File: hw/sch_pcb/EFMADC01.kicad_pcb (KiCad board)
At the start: 4 copper layers, 80 x 80 mm, 89 parts, among them J1 SM06B-GHS-TB, J2 SM03B-GHS-TB, J3 HEADER_1x01, J4 HEADER_2x03, J5 SM08B-GHS-TB, J6 SM06B-GHS-TB, SW1 KMT031 NGJ LHS C&K, U1 ISL21080DIH312Z-TK 1V25, U10 SN74LVC1G14QDCKRQ1, U11 SN74LVC1G14QDCKRQ1, U12 SN74LVC1G14QDCKRQ1, U13 VCNT2020, U2 OPA314, U3 MIC5504-3.3YM5, U4 PCF8583, U5 VCNT2020, U6 VCNT2020, U7 SHT31, U8 ATMEGA1284P-AU, U9 AT24CS64-SSHM, Y1 16MHz

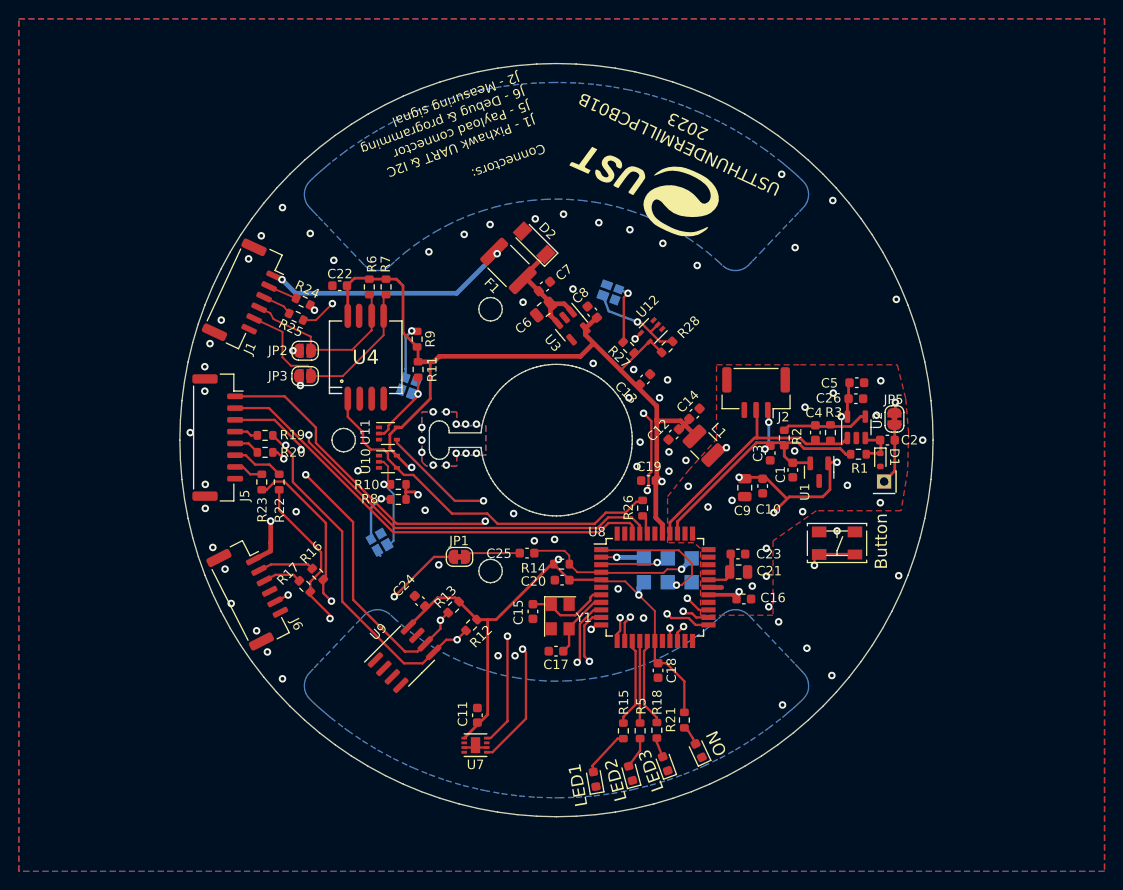
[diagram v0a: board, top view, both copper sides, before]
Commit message: Starting layout work.
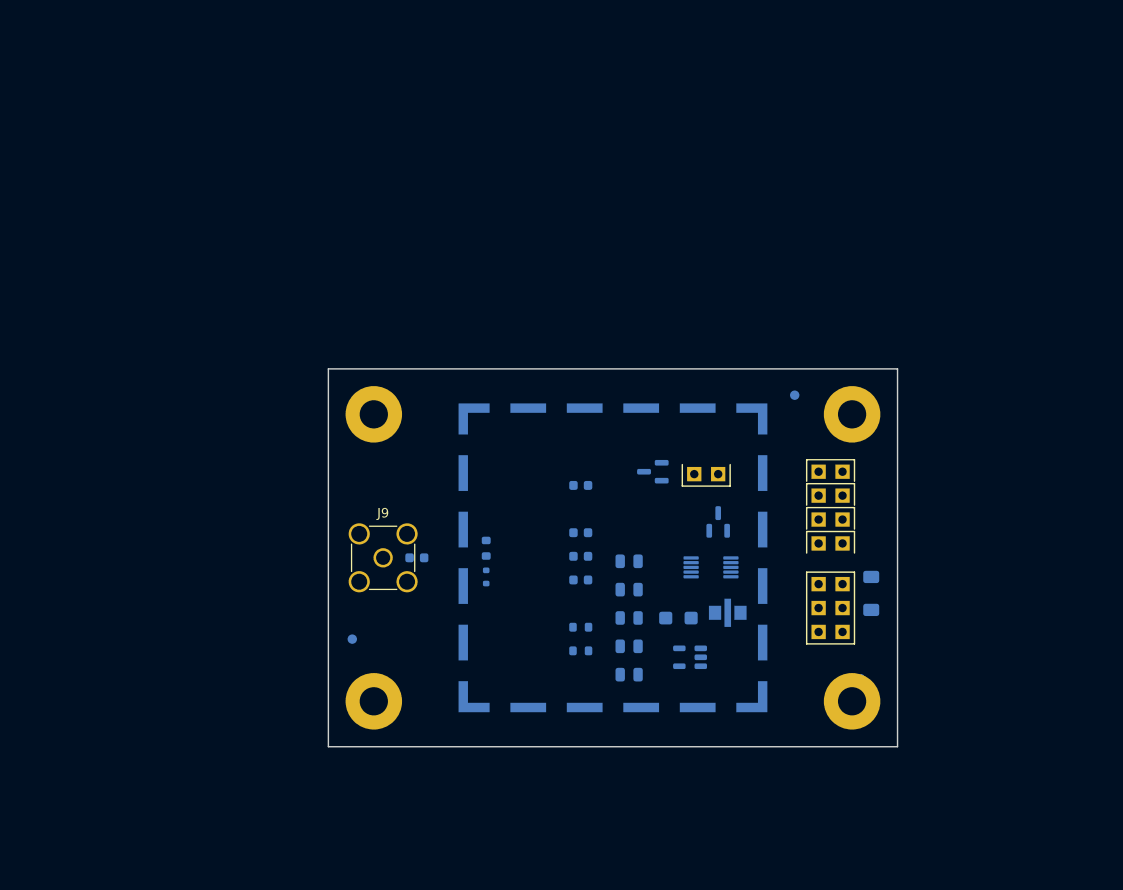
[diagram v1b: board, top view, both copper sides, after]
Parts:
- removed C13, C14, C16, C18, C19, C20, C22, C23, C24, C26: 100nF, Capacitor_SMD:C_0603_1608Metric
- removed C15, C17: 15 pF, Capacitor_SMD:C_0603_1608Metric
- removed C21: 10uF, Capacitor_SMD:C_0805_2012Metric
- removed C25: 4u7, Capacitor_SMD:C_0603_1608Metric
- removed D3: YELLOW, LED_SMD:LED_0603_1608Metric
- removed D4: BLUE, LED_SMD:LED_0603_1608Metric
- removed D5: GREEN, LED_SMD:LED_0603_1608Metric
- removed D6: RED, LED_SMD:LED_0603_1608Metric
- removed F1: 350mA, Fuse:Fuse_1812_4532Metric
- removed G1, G2: , MLAB_LOGA:UST
- removed J3: HEADER_1x01, Mlab_Pin_Headers:Straight_1x01
- removed JP2, JP3: SolderJumper_2_Open, Jumper:SolderJumper-2_P1.3mm_Open_RoundedPad1.0x1.5mm
- removed JP4: Jumper_2_Bridged, NetTie:NetTie-2_SMD_Pad0.5mm
- removed JP5: SolderJumper_2_Bridged, Jumper:SolderJumper-2_P1.3mm_Bridged_RoundedPad1.0x1.5mm
- removed L1: 10uH - LQH32CN100K23L, Inductor_SMD:L_1210_3225Metric
- removed R10, R11, R28: 4k7, Resistor_SMD:R_0603_1608Metric
- removed R12, R13, R14, R6, R7: 10k, Resistor_SMD:R_0603_1608Metric
- removed R15, R18, R21, R5: 2k2, Resistor_SMD:R_0603_1608Metric
- removed R16, R17, R22, R23, R24, R25, R26: 33R, Resistor_SMD:R_0603_1608Metric
- removed R19, R20, R27, R8, R9: 100R, Resistor_SMD:R_0603_1608Metric
- removed SW1: KMT031 NGJ LHS C&K, Mlab_SW:KMT031 NGJ LHS C&K
- removed U10, U11, U12: SN74LVC1G14QDCKRQ1, Package_TO_SOT_SMD:SOT-353_SC-70-5
- removed U13, U5, U6: VCNT2020, Mlab_IO:XDCR_VCNT2020
- removed U7: SHT31, Mlab_IO:DFN-8-1EP_2.4x2.4mm_Pitch0.5mm
- removed U8: ATMEGA1284P-AU, Package_QFP:TQFP-44_10x10mm_P0.8mm
- removed U9: AT24CS64-SSHM, Package_SO:SOIC-8_3.9x4.9mm_P1.27mm
- removed Y1: 16MHz, Mlab_XTAL:Crystal SMD CFPX-180
- added FID1: Fiducial, Fiducial:Fiducial_1mm_Mask2mm, B.Cu at (167.8, 87.7)
- added FID2: Fiducial, Fiducial:Fiducial_1mm_Mask2mm, B.Cu at (120.8, 113.6)
- added J7: HEADER_2x01_PARALLEL, Mlab_Pin_Headers:Straight_2x01, F.Cu at (171.6, 103.5)
- added J9: MCX, Connector_Coaxial:SMA_Amphenol_901-144_Vertical, F.Cu at (124.1, 105.0)
- added M1: RFShield_TwoPieces, RF_Shielding:Laird_Technologies_BMI-S-204-F_32.00x32.00mm, B.Cu at (148.5, 105.0)
- added M2: HOLE, Mlab_Mechanical:MountingHole_3mm, F.Cu at (123.1, 89.8)
- added M3: HOLE, Mlab_Mechanical:MountingHole_3mm, F.Cu at (173.9, 89.8)
- added M4: HOLE, Mlab_Mechanical:MountingHole_3mm, F.Cu at (123.1, 120.2)
- added M5: HOLE, Mlab_Mechanical:MountingHole_3mm, F.Cu at (173.9, 120.2)
- C1, C2, C3, C4, C5, D1, R1, R2, R3, U1, U2: moved to B.Cu
- C10, C11, C12: footprint Capacitor_SMD:C_0603_1608Metric -> Capacitor_SMD:C_0805_2012Metric; moved to B.Cu
- C6: value 10uF -> 1uF; footprint Capacitor_SMD:C_0805_2012Metric -> Mlab_L:FIR_0805; moved to B.Cu
- C7: value 1uF -> 100nF; footprint Capacitor_SMD:C_0603_1608Metric -> Capacitor_SMD:C_0805_2012Metric; moved to B.Cu
- C8: value 1uF -> 10uF; footprint Capacitor_SMD:C_0603_1608Metric -> Capacitor_SMD:C_0805_2012Metric; moved to B.Cu
- C9: footprint Capacitor_SMD:C_0805_2012Metric -> Capacitor_Tantalum_SMD:CP_EIA-3216-18_Kemet-A; moved to B.Cu
- D2: value ZENER-6.2V -> BZV55C-6,2V; footprint Mlab_D:Diode-MiniMELF_Standard -> Diode_SMD:D_MiniMELF; moved to B.Cu
- J1: value SM06B-GHS-TB -> 3.3-5V; footprint Connector_JST:JST_GH_SM06B-GHS-TB_1x06-1MP_P1.25mm_Horizontal -> Mlab_Pin_Headers:Straight_2x03
- J2: value SM03B-GHS-TB -> HEADER_2x01; footprint Connector_JST:JST_GH_SM03B-GHS-TB_1x03-1MP_P1.25mm_Horizontal -> Mlab_Pin_Headers:Straight_2x01
- J4: value HEADER_2x03 -> HEADER_2x01_PARALLEL; footprint Mlab_Pin_Headers:SMD_2x03 -> Mlab_Pin_Headers:Straight_2x01; moved to F.Cu
- J5: value SM08B-GHS-TB -> HEADER_2x01_PARALLEL; footprint Connector_JST:JST_GH_SM08B-GHS-TB_1x08-1MP_P1.25mm_Horizontal -> Mlab_Pin_Headers:Straight_2x01
- J6: value SM06B-GHS-TB -> HEADER_2x01_PARALLEL; footprint Connector_JST:JST_GH_SM06B-GHS-TB_1x06-1MP_P1.25mm_Horizontal -> Mlab_Pin_Headers:Straight_2x01
- JP1: value SolderJumper_2_Bridged -> Jumper_2_Bridged; footprint Jumper:SolderJumper-2_P1.3mm_Bridged_RoundedPad1.0x1.5mm -> NetTie:NetTie-2_SMD_Pad0.5mm; moved to B.Cu
- U3: value MIC5504-3.3YM5 -> ISL21080CIH330Z-TK; footprint Package_TO_SOT_SMD:SOT-23-5 -> Package_TO_SOT_SMD:SOT-23; moved to B.Cu
- U4: value PCF8583 -> LTC1865-MS; footprint Mlab_IO:SOT176-1 -> Package_SO:MSOP-10_3x3mm_P0.5mm; moved to B.Cu
- moved J1 70.4 mm to (171.6, 110.3), turned to 0 degrees
- moved J5 65.4 mm to (171.6, 98.4), turned to 180 degrees
- moved J6 62.9 mm to (171.6, 95.9), turned to 180 degrees
- moved D2 51.7 mm to (175.9, 108.8), turned to 90 degrees
- moved C2 51.5 mm to (127.7, 105.0), turned to 0 degrees
- moved JP1 44.1 mm to (174.4, 117.6)
- moved D1 43.7 mm to (135.0, 107.0)
- moved U4 42.9 mm to (158.9, 106.0)
- moved R1 40.8 mm to (135.0, 104.0), turned to -90 degrees
- moved C6 37.7 mm to (160.7, 110.8), turned to 0 degrees
- moved C5 36.0 mm to (145.1, 107.4)
- moved R3 35.2 mm to (145.1, 114.9), turned to 180 degrees
- moved C7 30.5 mm to (150.2, 105.4), turned to 180 degrees
- moved U2 30.1 mm to (156.7, 115.6), turned to 180 degrees
- moved C8 29.7 mm to (150.2, 108.4), turned to 180 degrees
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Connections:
- C1 pad 1: PA1 -> /REF_1V25
- C10 pad 1: +3.3VA -> VCC
- C10 pad 2: GNDA -> GND
- C11 pad 1: +3V3 -> Net-(U4-V_{REF})
- C11 pad 2: GND -> GNDA
- C12 pad 1: +3V3 -> VCC
- C12 pad 2: GND -> GNDA
- C3 pad 2: PA1 -> /REF_1V25
- C4 pad 2: PA0 -> Net-(U4-CH0)
- C6 pad 1: Net-(D2-K) -> VCC
- C8 pad 1: +3V3 -> Net-(D2-K)
- C9 pad 1: +3.3VA -> VCC
- C9 pad 2: GNDA -> GND
- J1 pad 1: +5V -> GND
- J1 pad 2: Net-(J1-Pad2) -> GND
- J1 pad 3: Net-(J1-Pad3) -> Net-(D2-K)
- J1 pad 4: SCL_RPM -> Net-(D2-K)
- J1 pad 5: SDA_RPM -> GND
- J2 pad 1: PA1 -> Net-(U4-V_{REF})
- J2 pad 2: PA0 -> Net-(U3-Vout)
- J4 pad 1: /CPU/PB6 -> Net-(U4-SCK)
- J4 pad 2: +3V3 -> Net-(U4-SCK)
- J5 pad 1: /CPU/TIMEPULSE -> Net-(U4-SDO)
- J5 pad 2: /CPU/EXTINT -> Net-(U4-SDO)
- J6 pad 1: +5V -> Net-(U4-SDI)
- J6 pad 2: Net-(J6-Pad2) -> Net-(U4-SDI)
- JP1 pad 1: Net-(JP1-A) -> GNDA
- JP1 pad 2: Net-(JP1-B) -> GND
- R1 pad 1: PA1 -> /REF_1V25
- R2 pad 1: PA1 -> /REF_1V25
- R3 pad 2: PA0 -> Net-(U4-CH0)
- U1 pad 2: PA1 -> /REF_1V25
- U2 pad 1: PA0 -> Net-(U4-CH0)
- U3 pad 1: Net-(D2-K) -> VCC
- U3 pad 2: GND -> Net-(U3-Vout)
- U3 pad 3: Net-(D2-K) -> GNDA
- U4 pad 1: COUNT_1 -> Net-(U4-CONV)
- U4 pad 2: unconnected-(U4-OSCO-Pad2) -> Net-(U4-CH0)
- U4 pad 3: GND -> /REF_1V25
- U4 pad 4: GND -> GNDA
- U4 pad 5: SDA_RPM -> GND
- U4 pad 6: SCL_RPM -> Net-(U4-SDI)
- U4 pad 7: unconnected-(U4-#INT-Pad7) -> Net-(U4-SDO)
- U4 pad 8: +3V3 -> Net-(U4-SCK)
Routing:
- net +3V3: track 174.5 -> 0.00 mm, vias 5 -> 0
- net /CPU/PC0: track 88.6 -> 0.00 mm, vias 6 -> 0
- net /CPU/PC1: track 86.1 -> 0.00 mm, vias 5 -> 0
- net /CPU/TX1: track 61.4 -> 0.00 mm, vias 2 -> 0
- net +5V: track 56.5 -> 0.00 mm, vias 3 -> 0
- net /CPU/TIMEPULSE: track 55.7 -> 0.00 mm, vias 2 -> 0
- net /CPU/RX1: track 55.5 -> 0.00 mm, vias 2 -> 0
- net /CPU/RX0: track 53.7 -> 0.00 mm, vias 2 -> 0
- net /CPU/TX0: track 53.5 -> 0.00 mm, vias 2 -> 0
- net /CPU/GEO_STAT: track 51.8 -> 0.00 mm, vias 2 -> 0
- net /CPU/EXTINT: track 49.0 -> 0.00 mm
- net +3.3VA: track 44.7 -> 0.00 mm, vias 6 -> 0
- net COUNT_2: track 41.6 -> 0.00 mm, vias 2 -> 0
- net COUNT_1: track 39.9 -> 0.00 mm
- net COUNT_3: track 35.5 -> 0.00 mm, vias 4 -> 0
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- removed copper zone on B.Cu, net GND
- removed copper zone on F.Cu, net GND
- removed copper zone on In1.Cu, net GND
- removed copper zone on In2.Cu, net GND
- removed copper zone on F.Cu, net GNDA
- removed copper zone on In1.Cu, net GNDA
- removed copper zone on B.Cu, net STATOR
- removed copper zone on In1.Cu, net STATOR
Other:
- board size 80 x 80 mm -> 60.5 x 40.1 mm
- board text removed: "#RST PB7 PB6 GND PB5 3V3"
- board text removed: "Button"
- board text removed: "Connectors: J1 - Pixhawk UART & I2C J5 - Payload connector J6 - Debug & programming J2 - Measuring signal"
- board text removed: "Debug UART"
- board text removed: "LED1"
- board text removed: "LED2"
- board text removed: "LED3"
- board text removed: "ON"
- board text removed: "Payload"
- board text removed: "Pixhawk I2C & UART"
- board text removed: "USTTHUNDERMILLPCB01B 2023"
